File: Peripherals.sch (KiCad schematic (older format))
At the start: 7 parts, among them J1 Micro_SD_Card, J2 Conn_01x04, U1 IMX6UL_BGA289

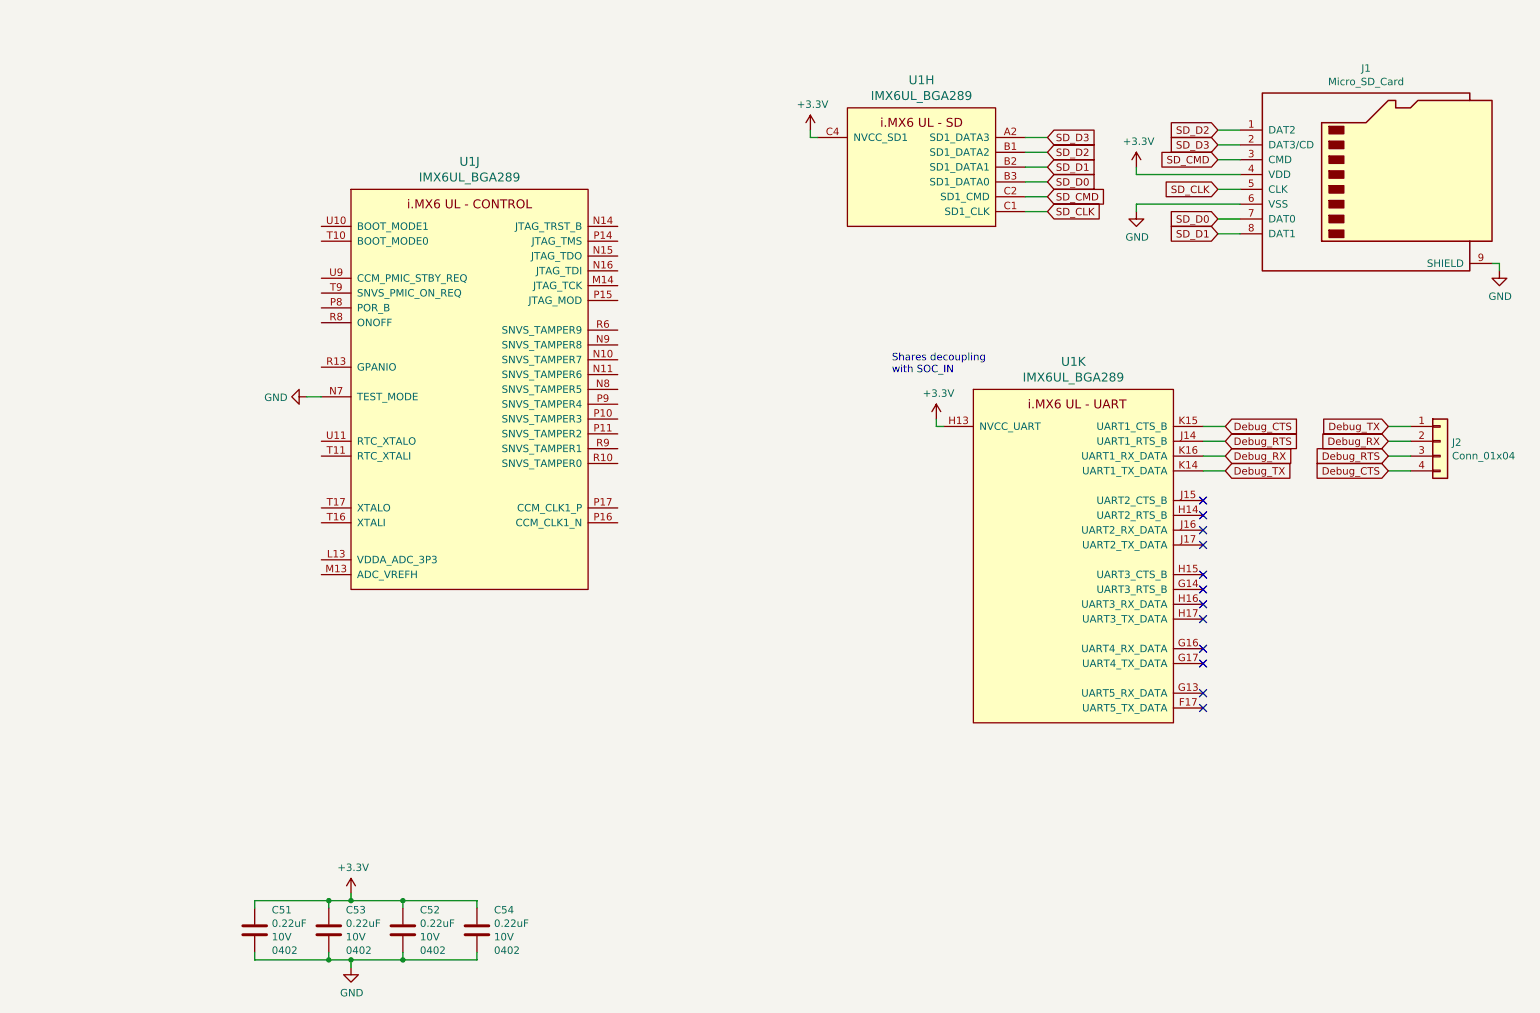
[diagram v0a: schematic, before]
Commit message: Finished first version of board
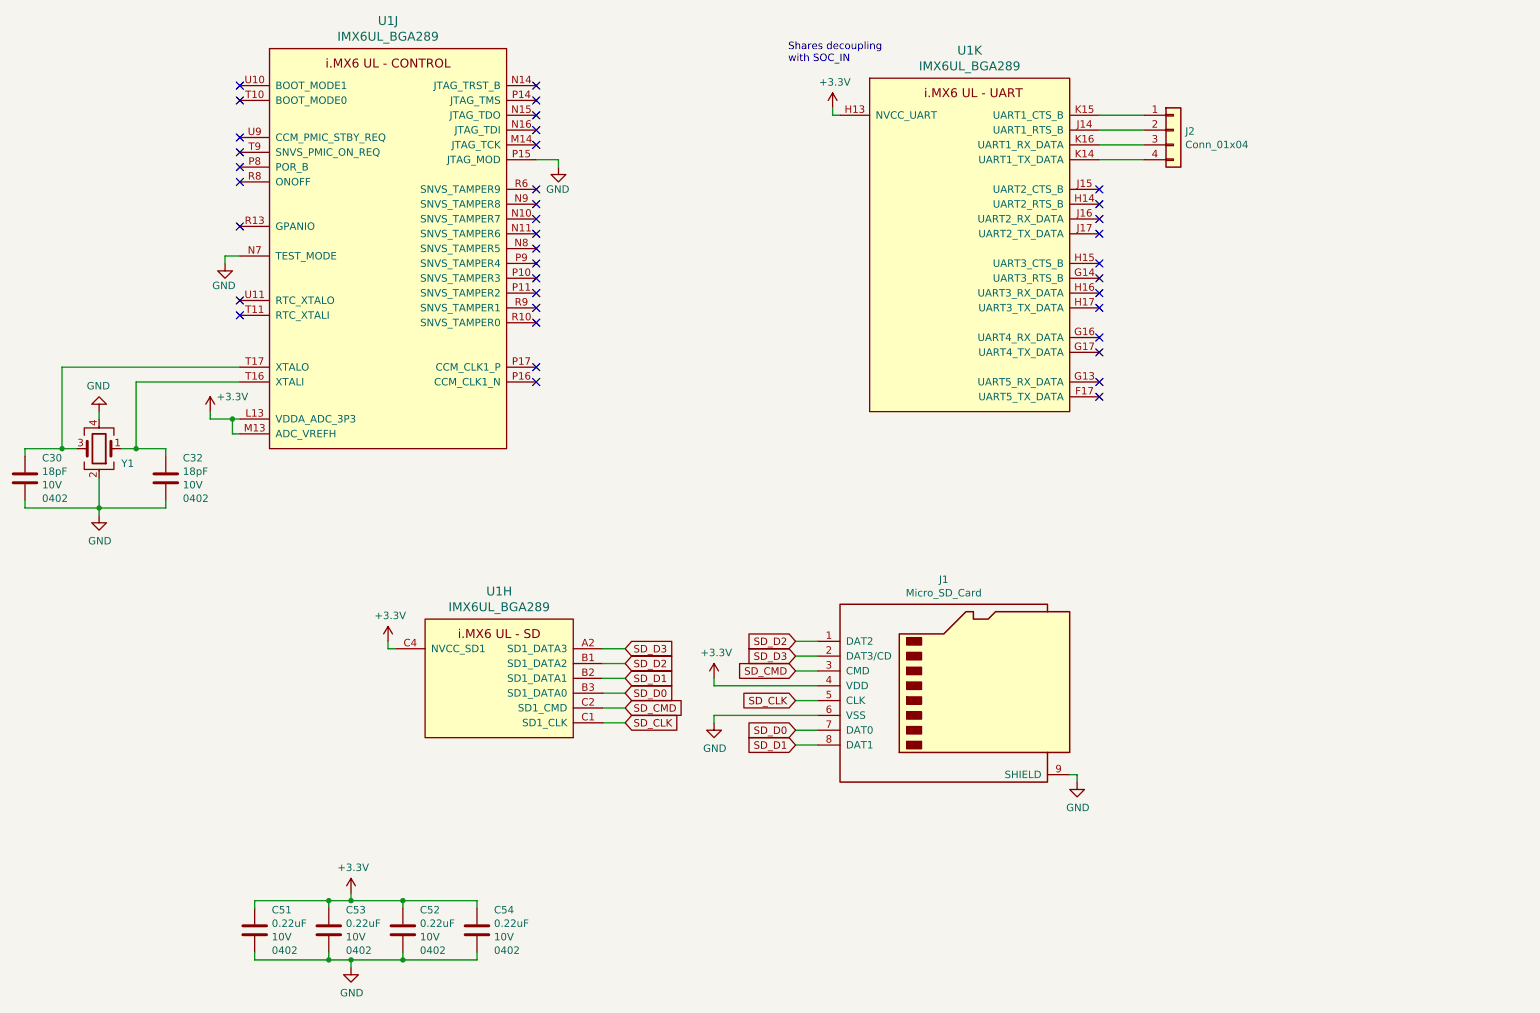
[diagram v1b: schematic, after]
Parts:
- added C30, C32: 18pF, Capacitor_SMD:C_0402_1005Metric, symbol Device:C
- added Y1: Crystal_GND24, Crystal:Crystal_SMD_3225-4Pin_3.2x2.5mm, symbol Device:Crystal_GND24
- C51, C52, C53, C54: LCSC (none) -> C16772
- U1: LCSC (none) -> C414042
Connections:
- net +3V3: now also U1.L13 (VDDA_ADC_3P3), U1.M13 (ADC_VREFH)
- net GND: now also U1.P15 (JTAG_MOD), C30.2, C32.2, Y1.2, Y1.4
- net at U1.T16 (XTALI): now also C32.1, Y1.1
- net at U1.T17 (XTALO): now also C30.1, Y1.3
- net Debug_CTS: no longer names the net of J2.4 (Pin_4)
- net Debug_CTS: now also U1.K14 (UART1_TX_DATA); no longer U1.K15 (UART1_CTS_B)
- net Debug_RTS: no longer names the net of U1.J14 (UART1_RTS_B)
- net Debug_RTS: now also J2.2 (Pin_2); no longer J2.3 (Pin_3)
- net Debug_RX: no longer names the net of U1.K16 (UART1_RX_DATA)
- net Debug_RX: now also J2.3 (Pin_3); no longer J2.2 (Pin_2)
- net Debug_TX: no longer names the net of J2.1 (Pin_1)
- net Debug_TX: now also U1.K15 (UART1_CTS_B); no longer U1.K14 (UART1_TX_DATA)
- no-connect marks 12 -> 38
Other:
- moved on the sheet: J1, J2, U1H, U1J, U1K
